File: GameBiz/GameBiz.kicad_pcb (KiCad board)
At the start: 2 copper layers, 89 x 51 mm, 90 parts, among them J1 USB4155-03-C_REVA, M1 C0720B001F, Q1 PMCXB900UEZ, SW1 CUS-12TB, U1 W25Q128JV, U2 RP2040, U3 NCV8718BMT330TBG, U4 BQ25172DSGR, U5 74LVC1G3157FZ4-7, U6 NRF24L01, U7 IQS7222A001QNR, U8 TPS61291DRVT, U9 EADOGS104NA, Y1 12MHz, Y2 ECS-160-18-30B-JEM-TR

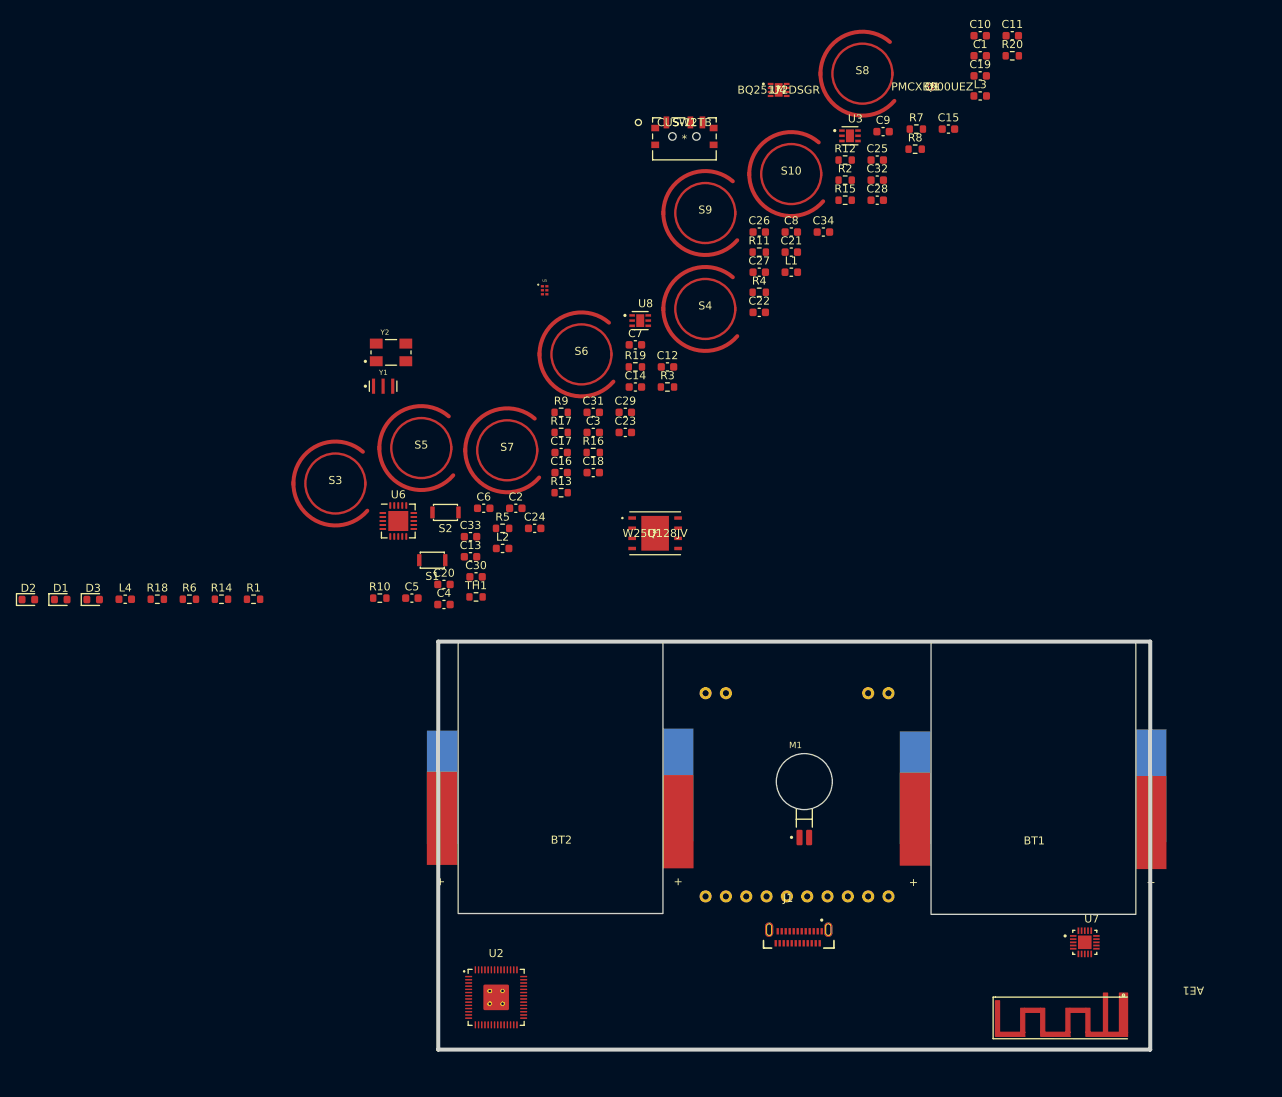
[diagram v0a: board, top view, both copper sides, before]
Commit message: layout almost finished
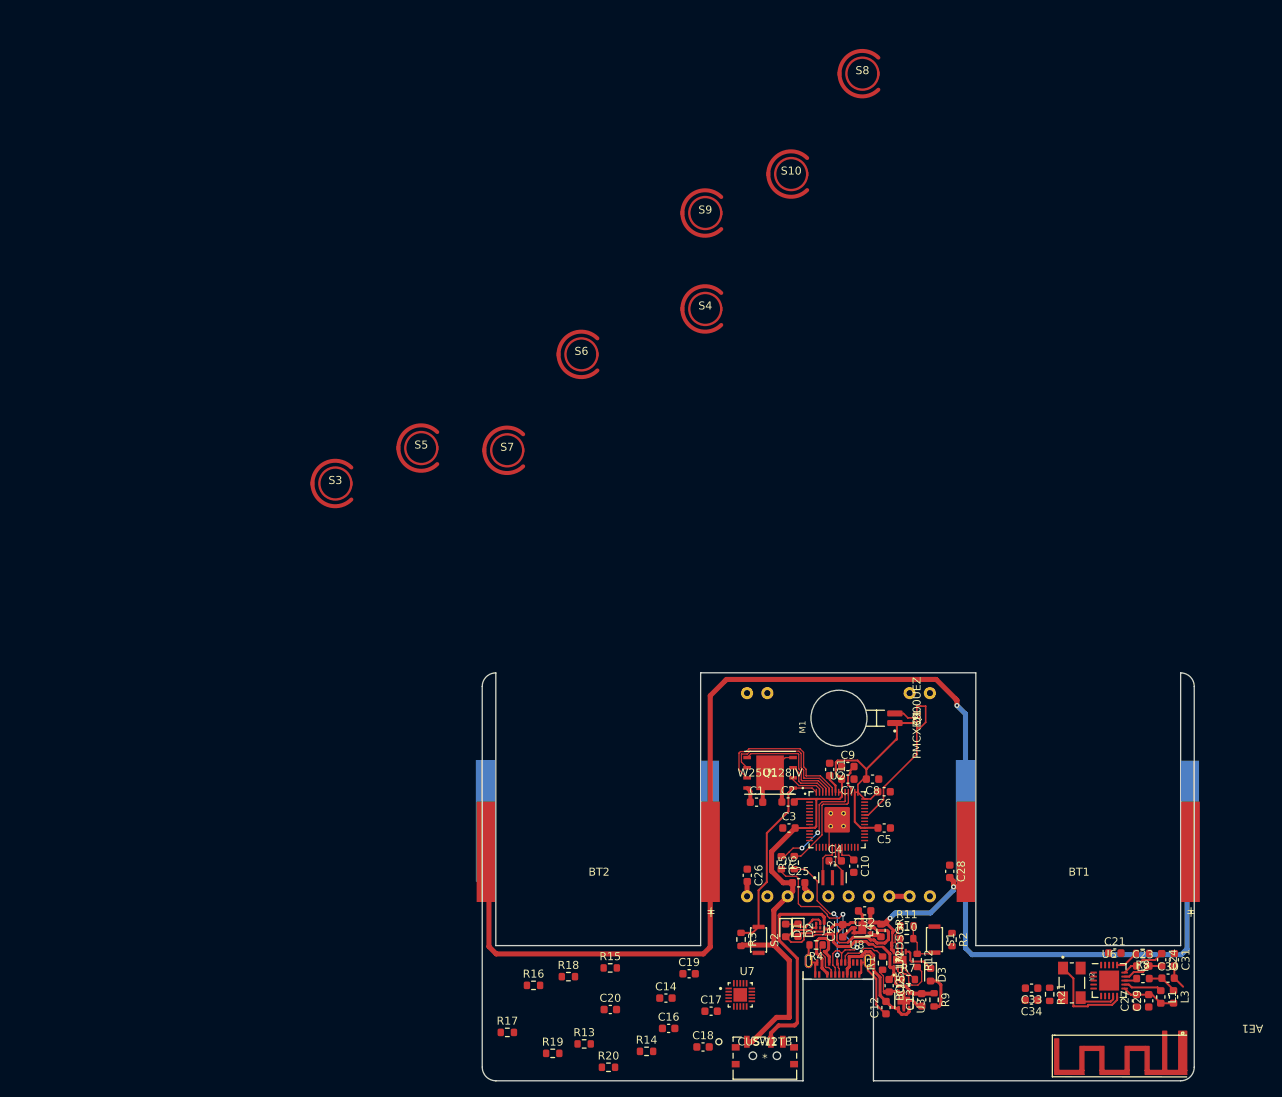
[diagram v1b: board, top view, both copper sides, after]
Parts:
- removed TH1: Thermistor, Resistor_SMD:R_0603_1608Metric
- added R12: 10K, Resistor_SMD:R_0603_1608Metric, F.Cu at (159.9, 139.8)
- moved C19 118.0 mm to (131.4, 141.5)
- moved R21 117.4 mm to (176.4, 144.1), turned to -90 degrees
- moved Y2 116.0 mm to (179.2, 142.7), turned to -90 degrees
- moved SW1 115.4 mm to (140.8, 152.1)
- moved R13 115.2 mm to (118.2, 150.3)
- moved L3 115.2 mm to (191.9, 144.4), turned to -90 degrees
- moved D3 114.7 mm to (161.5, 141.6), turned to -90 degrees
- moved U4 109.8 mm to (157.7, 139.8), turned to 90 degrees
- moved U3 108.3 mm to (158.2, 144.9), turned to -90 degrees
- moved C15 107.3 mm to (156.4, 143.0), turned to -90 degrees
- moved R7 106.3 mm to (158.8, 142.2)
- moved U6 105.8 mm to (183.9, 142.4)
- moved R16 105.6 mm to (111.9, 143.0)
- moved C10 105.0 mm to (151.9, 128.1), turned to -90 degrees
- moved D2 104.7 mm to (145.0, 136.1), turned to -90 degrees
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- renumbered R12 to R13, R13 to R14, R14 to R15, R15 to R16, R16 to R17, R17 to R18, R18 to R19, R19 to R20, R20 to R21
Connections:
- AE1 pad 1: GND -> Net-(AE1-Pad2)
- AE1 pad 2: Net-(AE1-Pad2) -> GND
- D2 pad 1: unconnected-(D2-Pad1) -> Net-(D1-Pad1)
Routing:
- net Net-(BT1-Pad2): track 0.00 -> 180.5 mm, vias 0 -> 1
- net +3.3V: track 0.00 -> 94.4 mm
- net GND: track 0.00 -> 66.3 mm
- net Net-(C13-Pad2): track 0.00 -> 31.8 mm
- net Net-(C12-Pad2): track 0.00 -> 26.4 mm
- net Net-(BT1-Pad1): track 0.00 -> 26.1 mm, vias 0 -> 2
- net Net-(SW1-Pad2): track 0.00 -> 25.9 mm
- net Net-(J1-PadA6): track 0.00 -> 25.0 mm, vias 0 -> 2
- net Net-(R3-Pad1): track 0.00 -> 24.8 mm
- net Net-(C22-Pad2): track 0.00 -> 20.9 mm
- net Net-(Q1-Pad2): track 0.00 -> 19.9 mm
- net Net-(U1-Pad7): track 0.00 -> 19.5 mm
- net Net-(U1-Pad6): track 0.00 -> 17.2 mm
- net Net-(J1-PadA7): track 0.00 -> 16.6 mm, vias 0 -> 2
- net Net-(U1-Pad5): track 0.00 -> 14.0 mm
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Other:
- outline, holes or cut-outs redrawn
